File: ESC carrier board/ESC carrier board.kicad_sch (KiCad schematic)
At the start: 11 parts, among them J1 Conn_01x04_Pin, J3 Conn_01x04_Pin, J4 Conn_01x04_Pin, U1 ESC, U2 ESC, U3 ESC

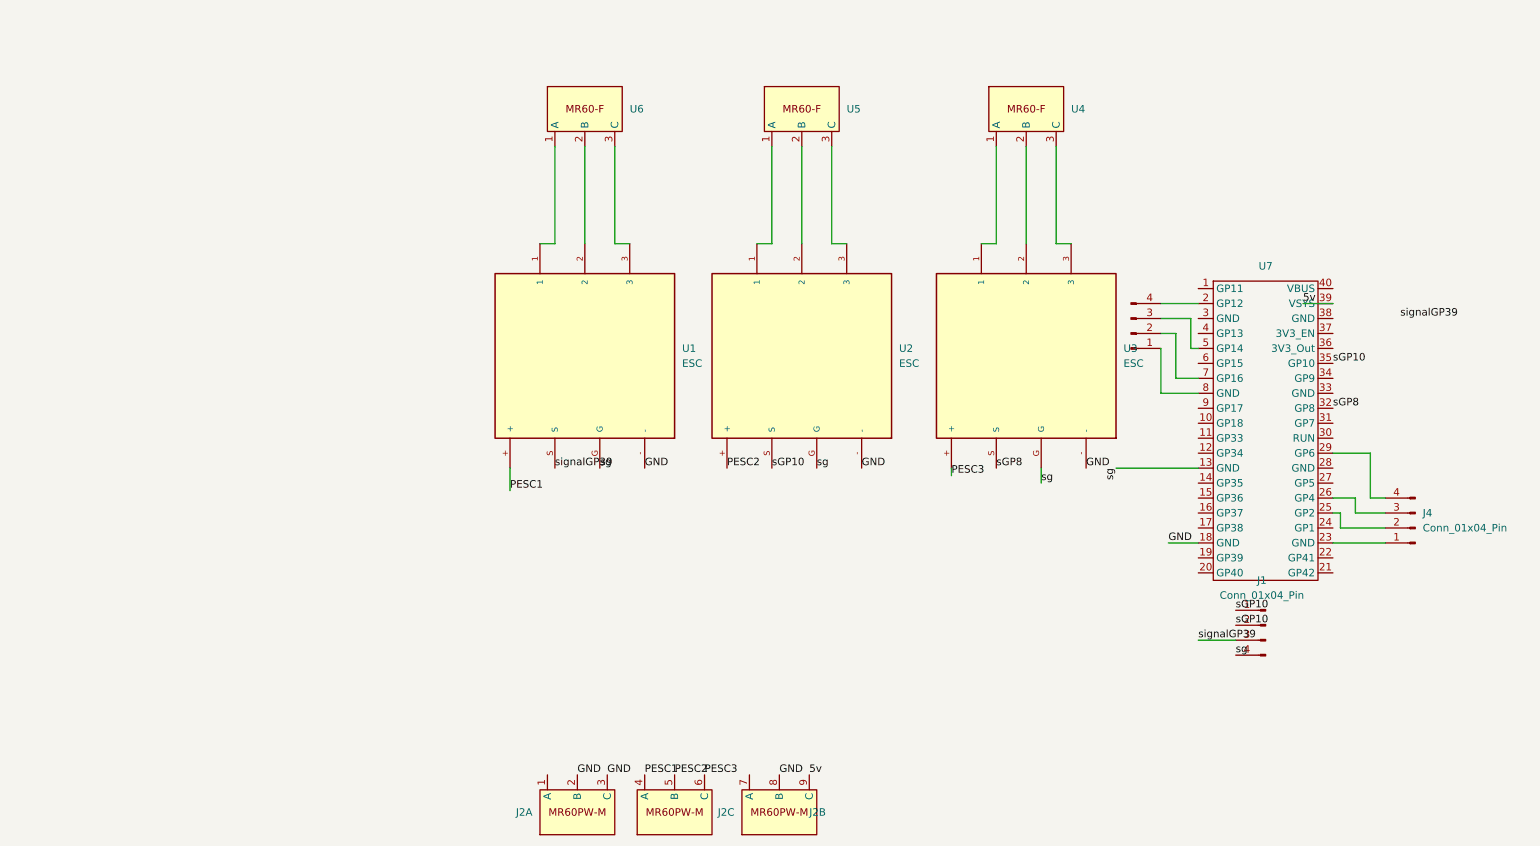
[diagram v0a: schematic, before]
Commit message: Partially cleaned up schematic
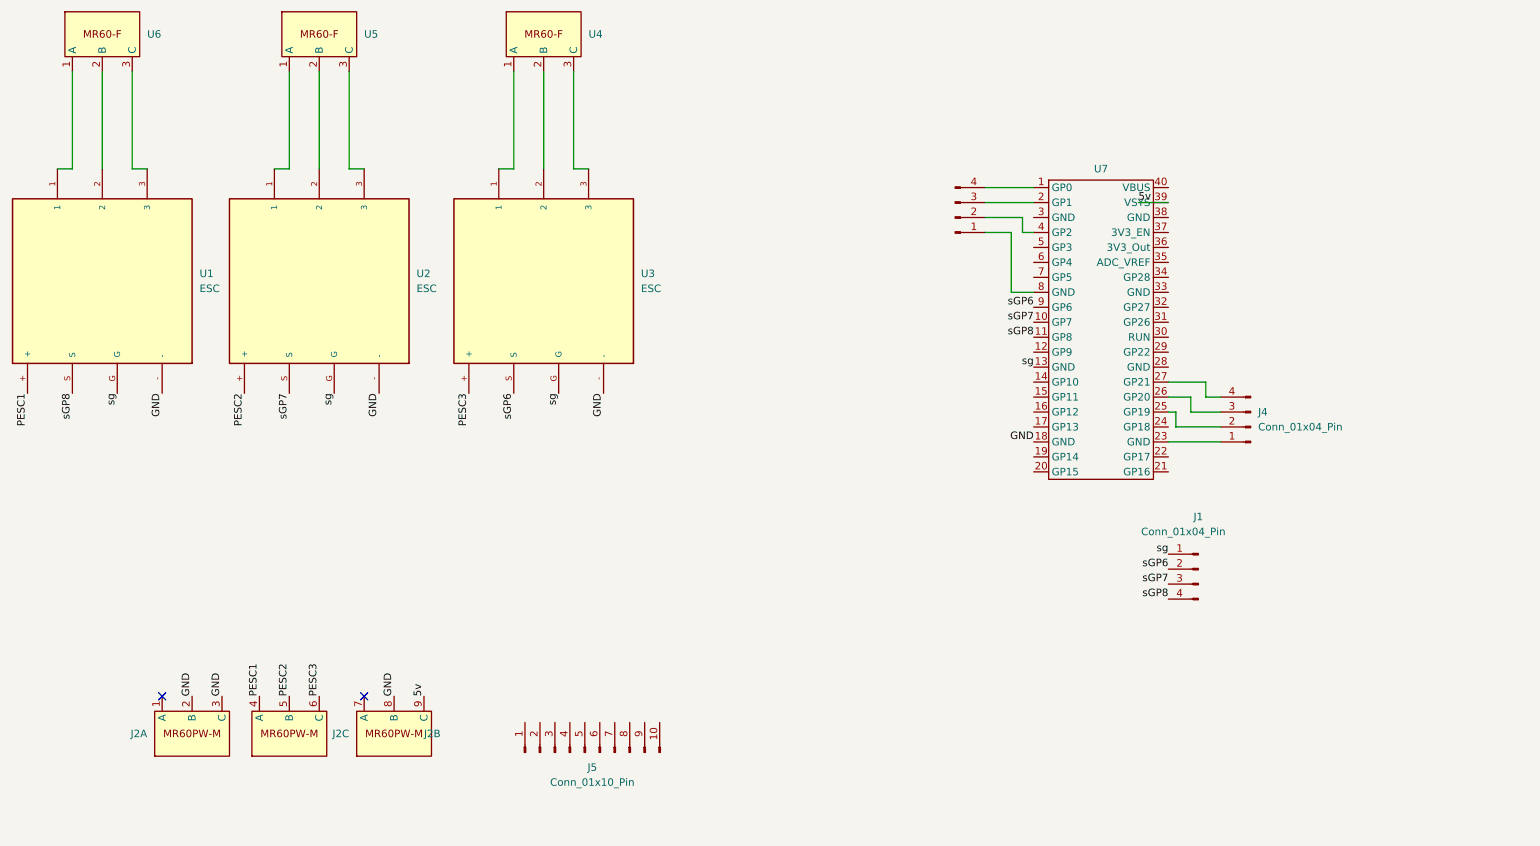
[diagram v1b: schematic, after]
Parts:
- added J5: Conn_01x10_Pin, symbol Connector:Conn_01x10_Pin
- J2: footprint ESC carrier board test 1:MR60PW-M_X3 -> 2024-backplane:MR60PW-M_X3
- U1: footprint ESC carrier board test 1:ESC -> ESC:ESC
- U7: symbol Kelpie_Library:ESP32-S3-Pico -> Kelpie_Library:Raspberry-Pi-Pico
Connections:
- net sGP8: now also J1.4 (Pin_4), U1.S, U7.11 (GP8); no longer U3.S, U7.32 (GP8)
- net sg: now also J1.1 (Pin_1); no longer J1.4 (Pin_4)
- net at J4.4 (Pin_4): now also U7.27 (GP21); no longer U7.29 (GP6)
- net at J3.2 (Pin_2): now also U7.4 (GP2); no longer U7.7 (GP16)
- net at J3.3 (Pin_3): now also U7.2 (GP1); no longer U7.5 (GP14)
- net at J3.4 (Pin_4): now also U7.1 (GP0); no longer U7.2 (GP12)
- net sGP7: now reaches U7.10 (GP7)
- net sGP7: now also J1.3 (Pin_3), U2.S
- net sGP6: now reaches U7.9 (GP6)
- net sGP6: now also J1.2 (Pin_2), U3.S
- removed net sGP10: J1.1 (Pin_1), J1.2 (Pin_2), U2.S, U7.35 (GP10)
- removed net signalGP39: J1.3 (Pin_3), U1.S
- no-connect marks 0 -> 2
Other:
- moved on the sheet: J1, J2A, J2B, J2C, J4, U1, U2, U3, U4, U5, U6, U7
